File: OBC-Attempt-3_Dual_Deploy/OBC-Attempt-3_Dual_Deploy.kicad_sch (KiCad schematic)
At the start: 31 parts, among them J1 Bat, J2 Bat, J3 PWR, J4 DEBUG, J5 CAN Header, SW1 SW_SPDT, SW2 SW_SPST, U1 LD1117S33TR_SOT223, U2 STM32F042G4Ux, U3 SN65HVD230, U4 MS560702BA03-50, U5 BMI088, U6 MMC5983MA, X1 ECS-2520MV-xxx-xx

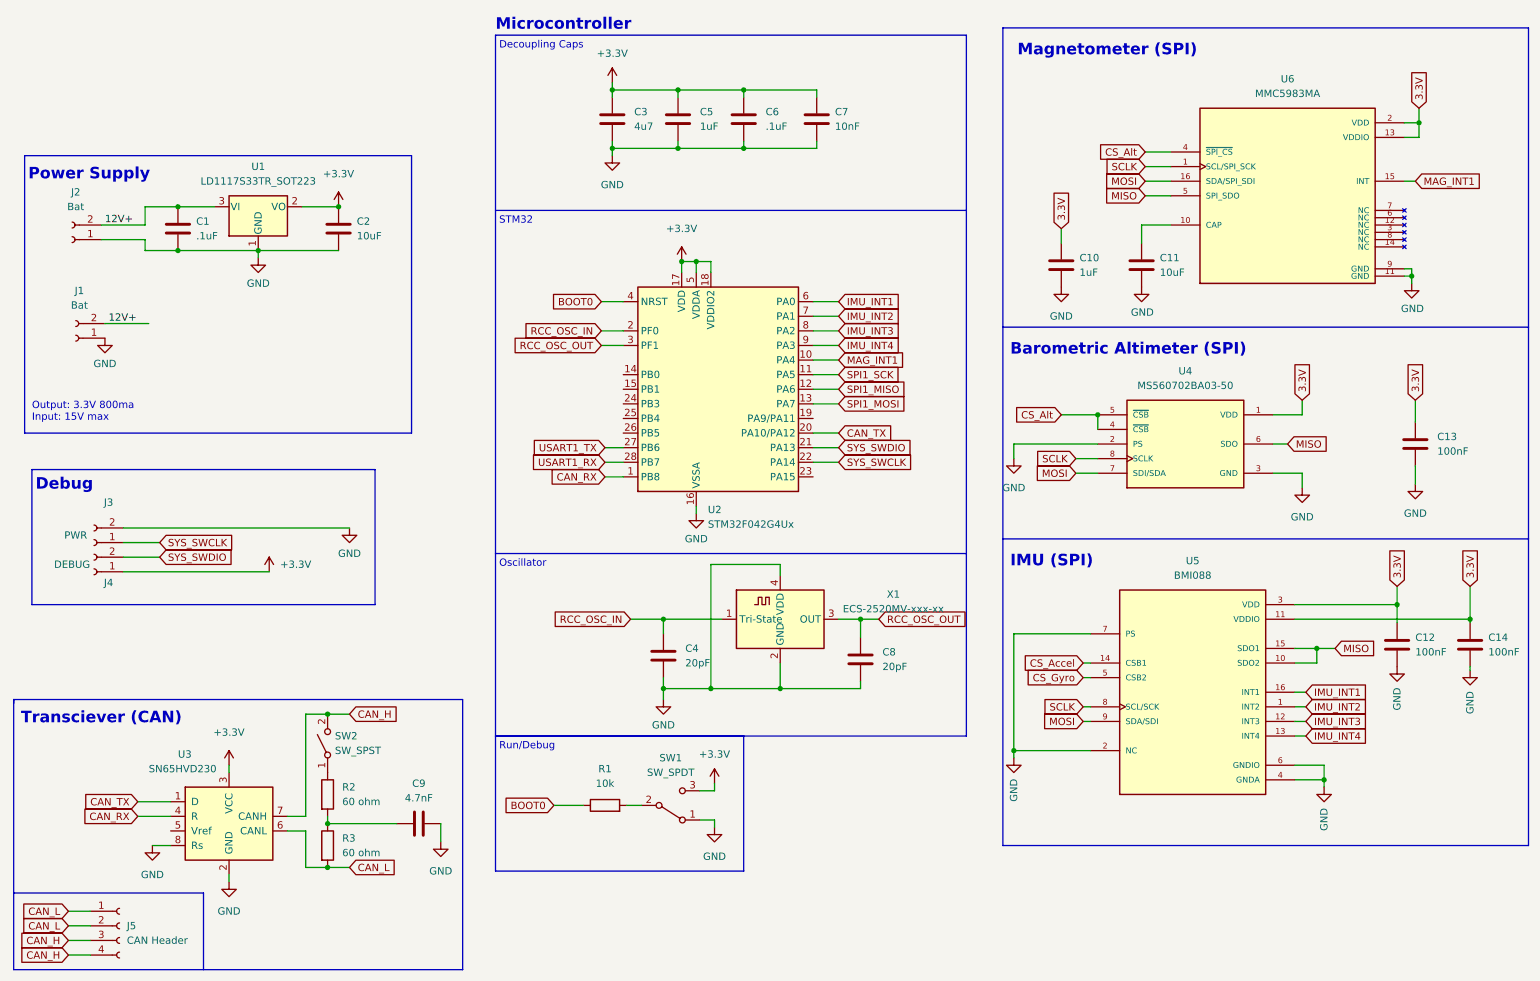
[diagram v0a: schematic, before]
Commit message: Re org da files
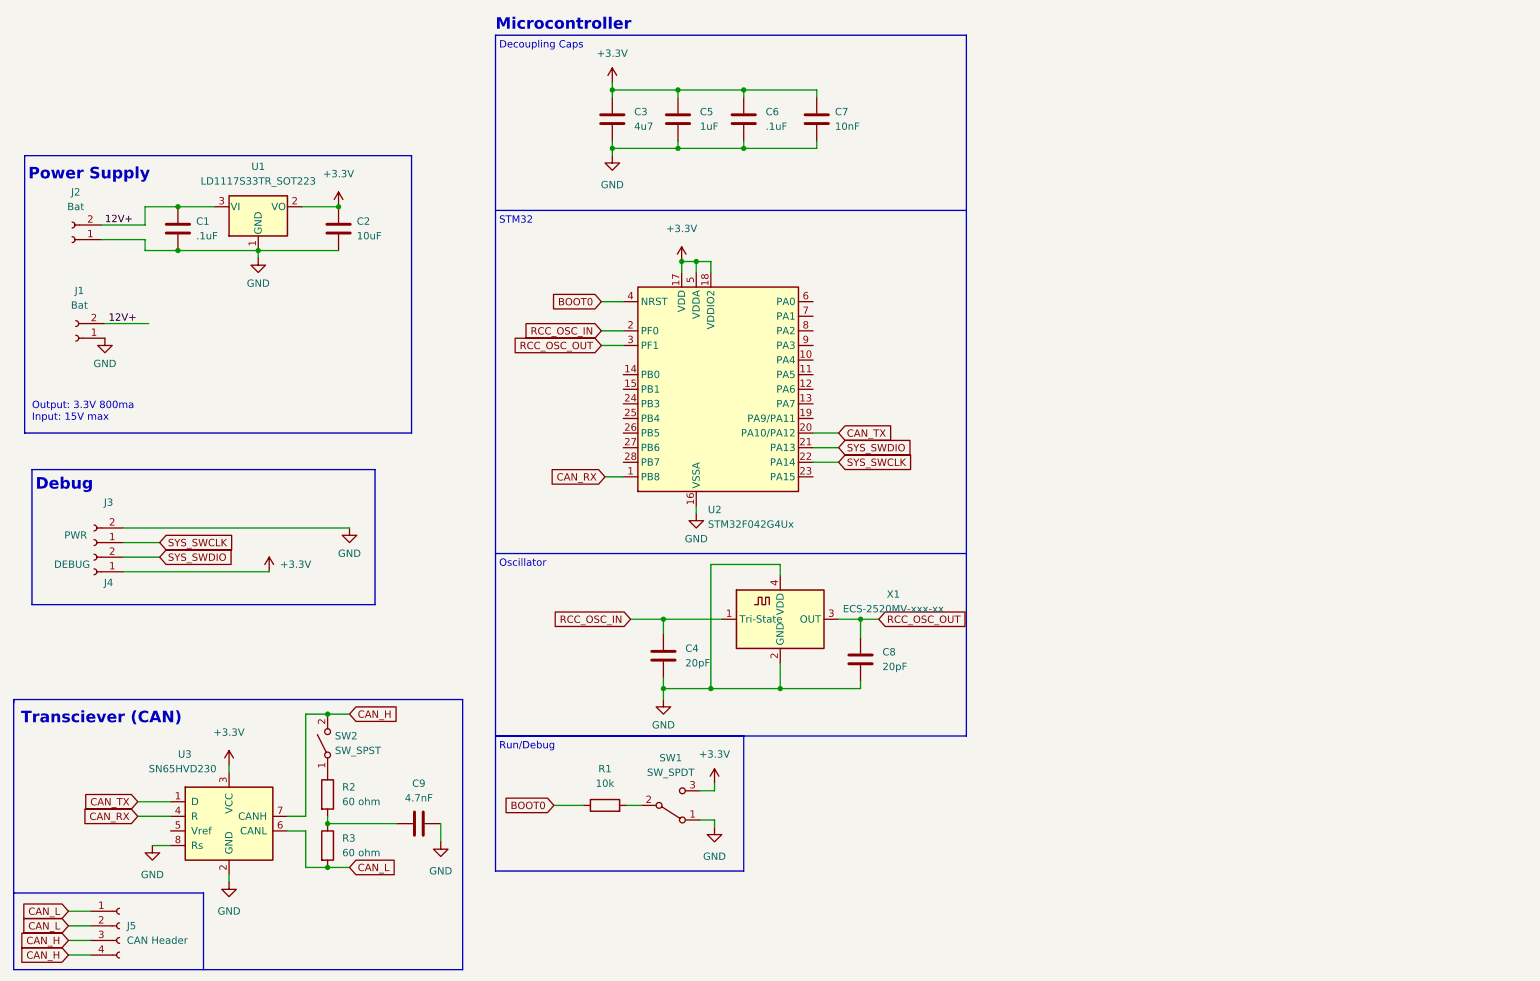
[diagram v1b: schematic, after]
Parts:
- removed C10: 1uF, Capacitor_SMD:C_0402_1005Metric, symbol Device:C
- removed C11: 10uF, Capacitor_SMD:C_0402_1005Metric, symbol Device:C
- removed C12, C13, C14: 100nF, Capacitor_SMD:C_0402_1005Metric, symbol Device:C
- removed U4: MS560702BA03-50, MS5607:SON125P300X500X100-8N, symbol MS5607-02BA03:MS560702BA03-50
- removed U5: BMI088, BMI088:PQFN50P450X300X100-16N, symbol BMI088:BMI088
- removed U6: MMC5983MA, MMC5983MA:PQFN50P300X300X100-16N, symbol MMC5983MA:MMC5983MA
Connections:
- net IMU_INT1: no longer names the net of U2.6 (PA0)
- net IMU_INT2: no longer names the net of U2.7 (PA1)
- net IMU_INT3: no longer names the net of U2.8 (PA2)
- net IMU_INT4: no longer names the net of U2.9 (PA3)
- net MAG_INT1: no longer names the net of U2.10 (PA4)
- net SPI1_MISO: no longer names the net of U2.12 (PA6)
- net SPI1_MOSI: no longer names the net of U2.13 (PA7)
- net SPI1_SCK: no longer names the net of U2.11 (PA5)
- net USART1_RX: no longer names the net of U2.28 (PB7)
- net USART1_TX: no longer names the net of U2.27 (PB6)
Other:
- note removed: "Barometric Altimeter (SPI)"
- note removed: "IMU (SPI)"
- note removed: "Magnetometer (SPI)"
